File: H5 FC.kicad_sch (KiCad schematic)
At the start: 0 parts

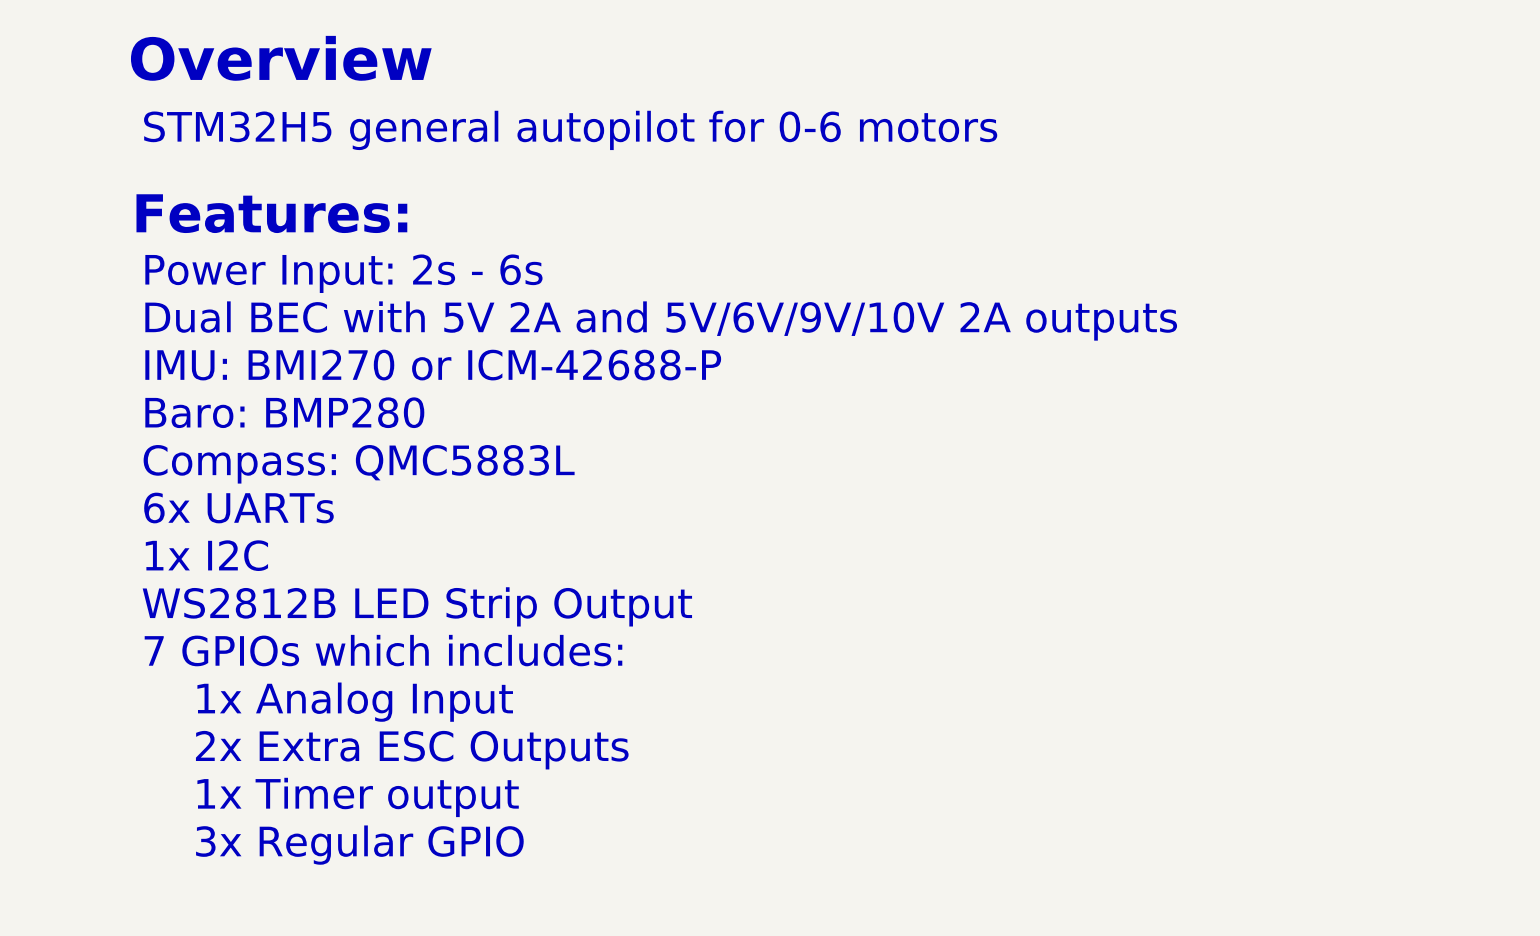
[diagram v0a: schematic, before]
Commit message: Add README
Add README

Add README

Add README

Add README
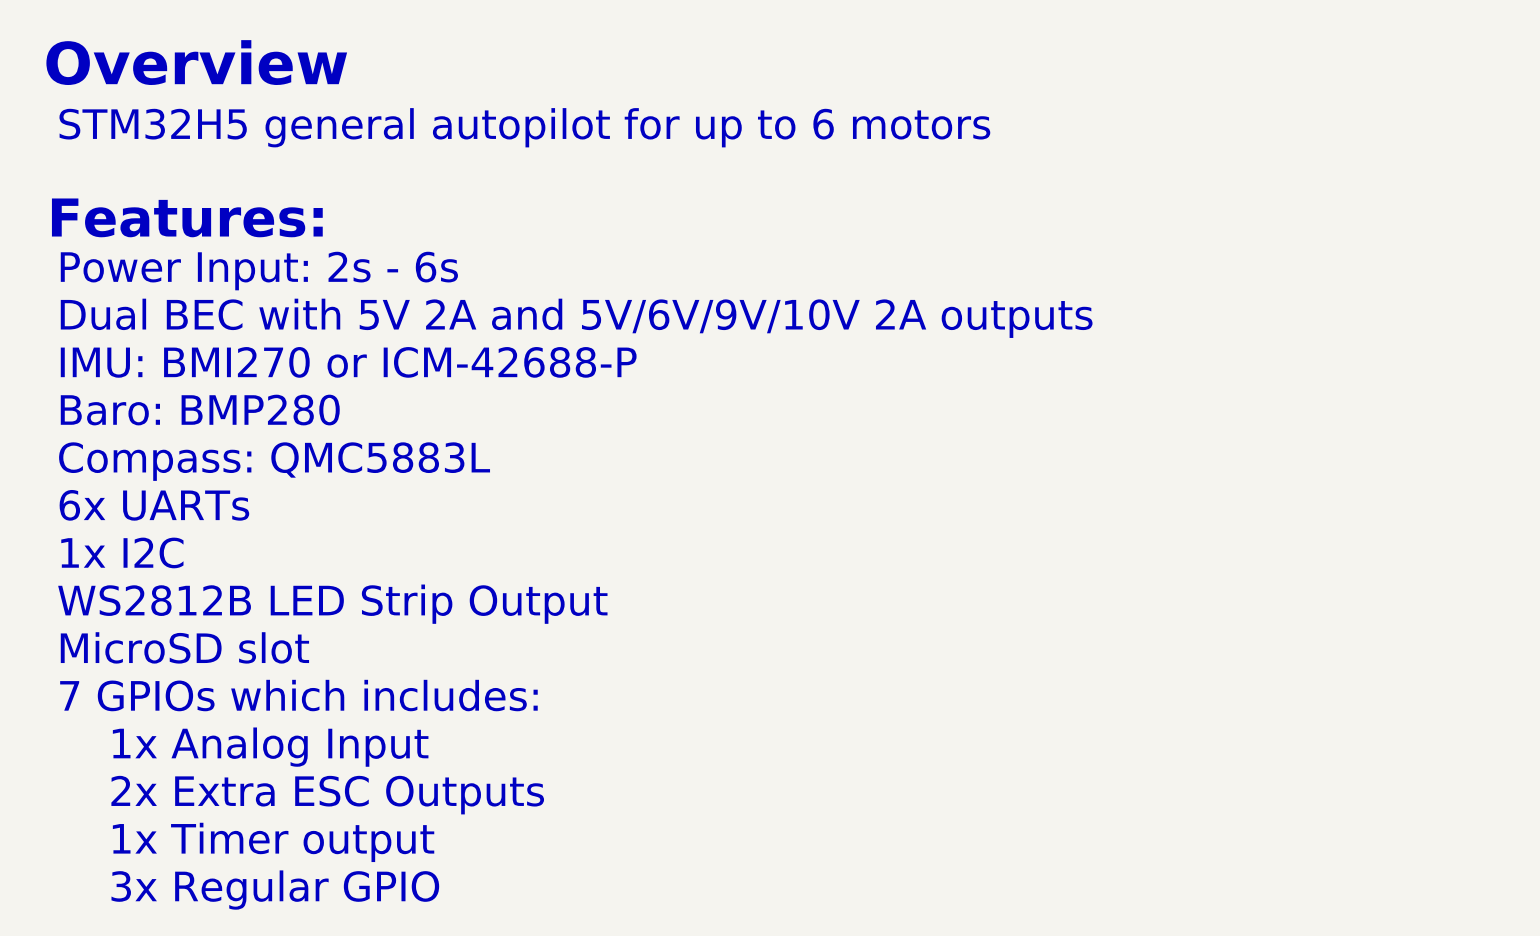
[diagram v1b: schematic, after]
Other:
- note added: "STM32H5 general autopilot for up to 6 motors Power Input: 2s - 6s Dual BEC with 5V 2A and 5V/6V/9V/10V 2A outputs IMU: BMI270 or ICM-42688-P Baro: BMP280 Compass: QMC5883L 6x UARTs 1x I2C WS2812B LED Strip Output MicroSD slot 7 GPIOs which includes: 1x Analog Input 2x Extra ESC Outputs 1x Timer output 3x Regular GPIO"
- note removed: "STM32H5 general autopilot for 0-6 motors Power Input: 2s - 6s Dual BEC with 5V 2A and 5V/6V/9V/10V 2A outputs IMU: BMI270 or ICM-42688-P Baro: BMP280 Compass: QMC5883L 6x UARTs 1x I2C WS2812B LED Strip Output 7 GPIOs which includes: 1x Analog Input 2x Extra ESC Outputs 1x Timer output 3x Regular GPIO"
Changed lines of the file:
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@@
 	(text "Overview"
 		(exclude_from_sim no)
-		(at 106.172 55.372 0)
+		(at 96.012 55.88 0)
 		(effects
 			(font
@@
 	(text "Features:"
 		(exclude_from_sim no)
-		(at 105.156 73.914 0)
+		(at 94.996 74.422 0)
 		(effects
 			(font
@@
 		)
 	)
-	(text "STM32H5 general autopilot for 0-6 motors\n\n\nPower Input: 2s - 6s\nDual BEC with 5V 2A and 5V/6V/9V/10V 2A outputs\nIMU: BMI270 or ICM-42688-P\nBaro: BMP280\nCompass: QMC5883L\n6x UARTs\n1x I2C\nWS2812B LED Strip Output\n7 GPIOs which includes:\n	1x Analog Input\n	2x Extra ESC Outputs\n	1x Timer output\n	3x Regular GPIO "
+	(text "STM32H5 general autopilot for up to 6 motors\n\n\nPower Input: 2s - 6s\nDual BEC with 5V 2A and 5V/6V/9V/10V 2A outputs\nIMU: BMI270 or ICM-42688-P\nBaro: BMP280\nCompass: QMC5883L\n6x UARTs\n1x I2C\nWS2812B LED Strip Output\nMicroSD slot\n7 GPIOs which includes:\n	1x Analog Input\n	2x Extra ESC Outputs\n	1x Timer output\n	3x Regular GPIO "
 		(exclude_from_sim yes)
-		(at 89.408 106.426 0)
+		(at 79.248 108.966 0)
 		(effects
 			(font
